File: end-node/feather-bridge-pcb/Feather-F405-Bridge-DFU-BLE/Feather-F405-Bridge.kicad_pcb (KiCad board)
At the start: 2 copper layers, 38.8 x 52.4 mm, 14 parts, among them J1 Conn_01x06, J3 Conn_02x06_Odd_Even, SW1 SW_SPST, SW2 SW_SPST, U1 LoRa Radio FeatherWing, U2 NUD3112LT1, U3 NUD3112LT1

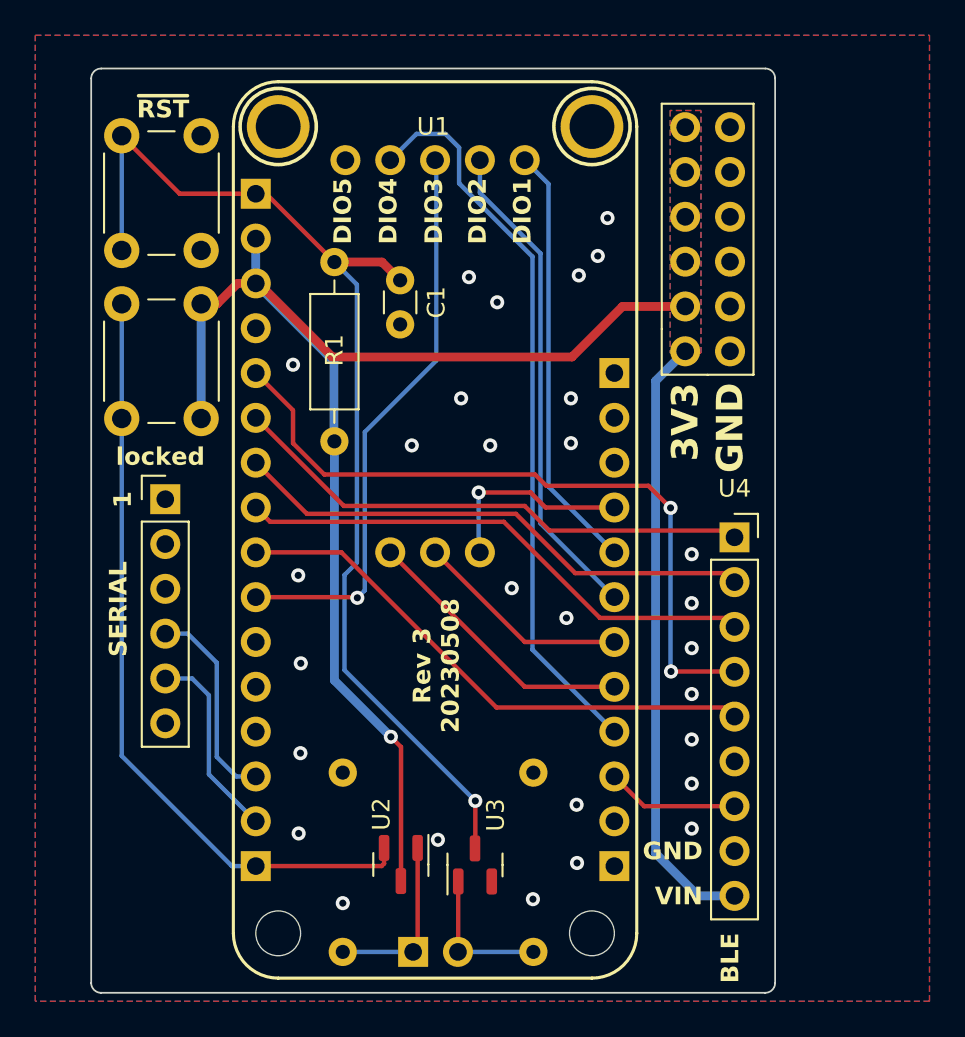
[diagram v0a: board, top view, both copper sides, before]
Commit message: misc aesthetic tweaks
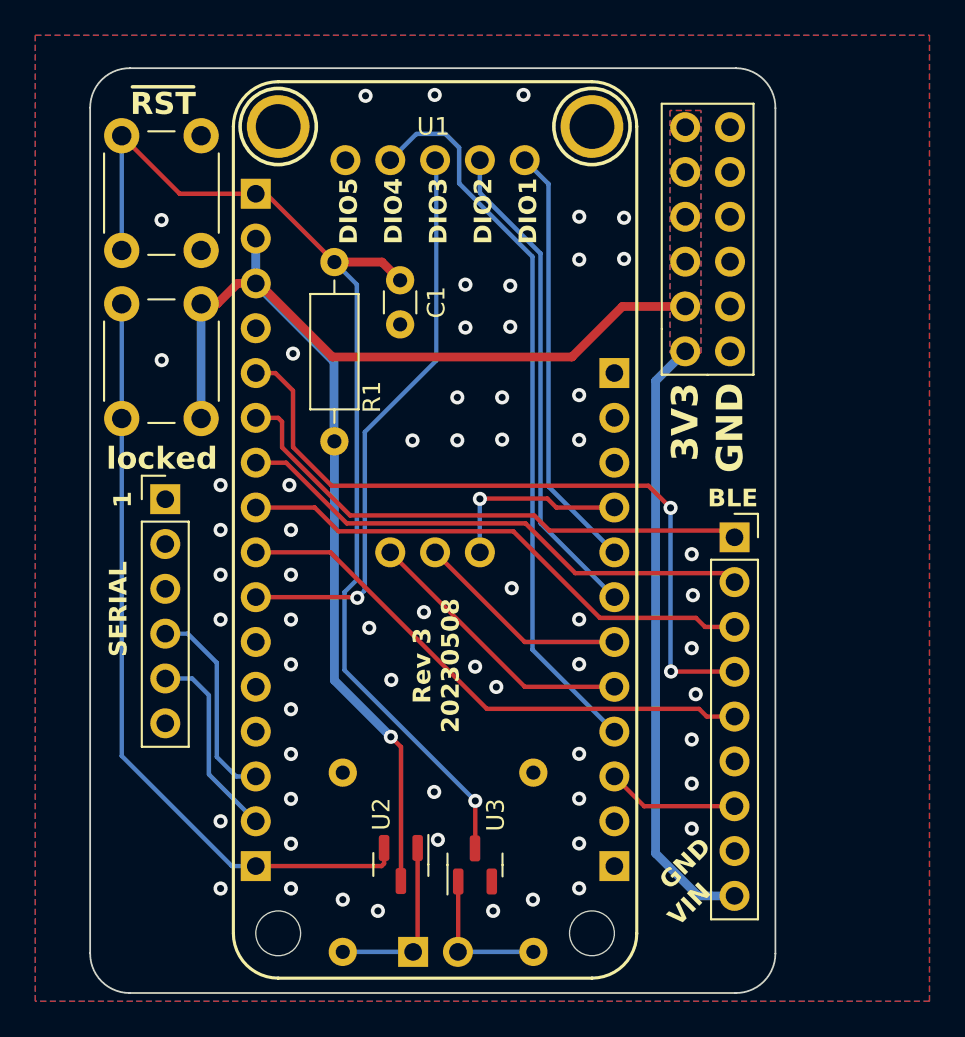
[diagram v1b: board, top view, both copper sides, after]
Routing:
- net BLUEFRUIT_SCK: track 29.9 -> 30.8 mm
- net BLUEFRUIT_CS: track 40.7 -> 41.4 mm
- net GND: vias 29 -> 62
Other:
- outline, holes or cut-outs redrawn
